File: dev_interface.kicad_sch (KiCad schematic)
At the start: 8 parts, among them U4 ISO164xB, U5 DACx53401, U6 DACx53401, U8 LM2904

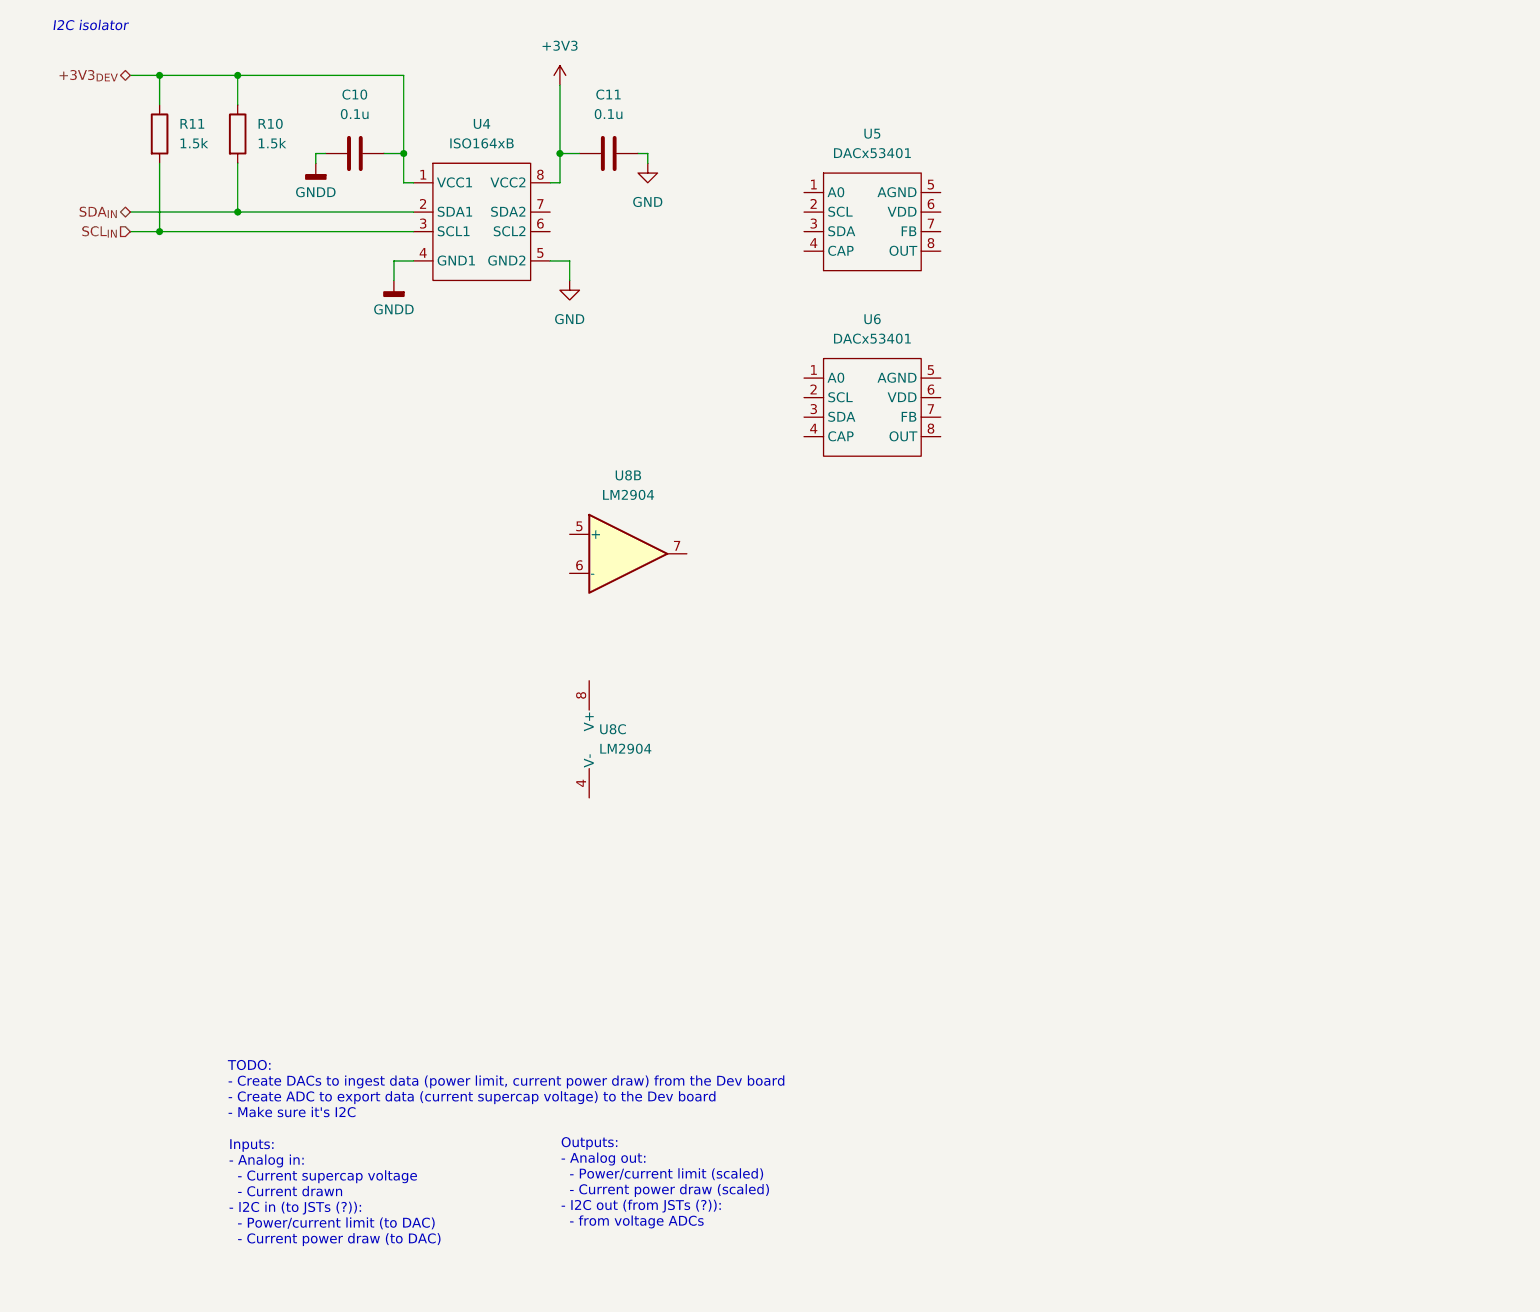
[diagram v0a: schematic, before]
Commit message: Finish Dev board interface
sorry morris
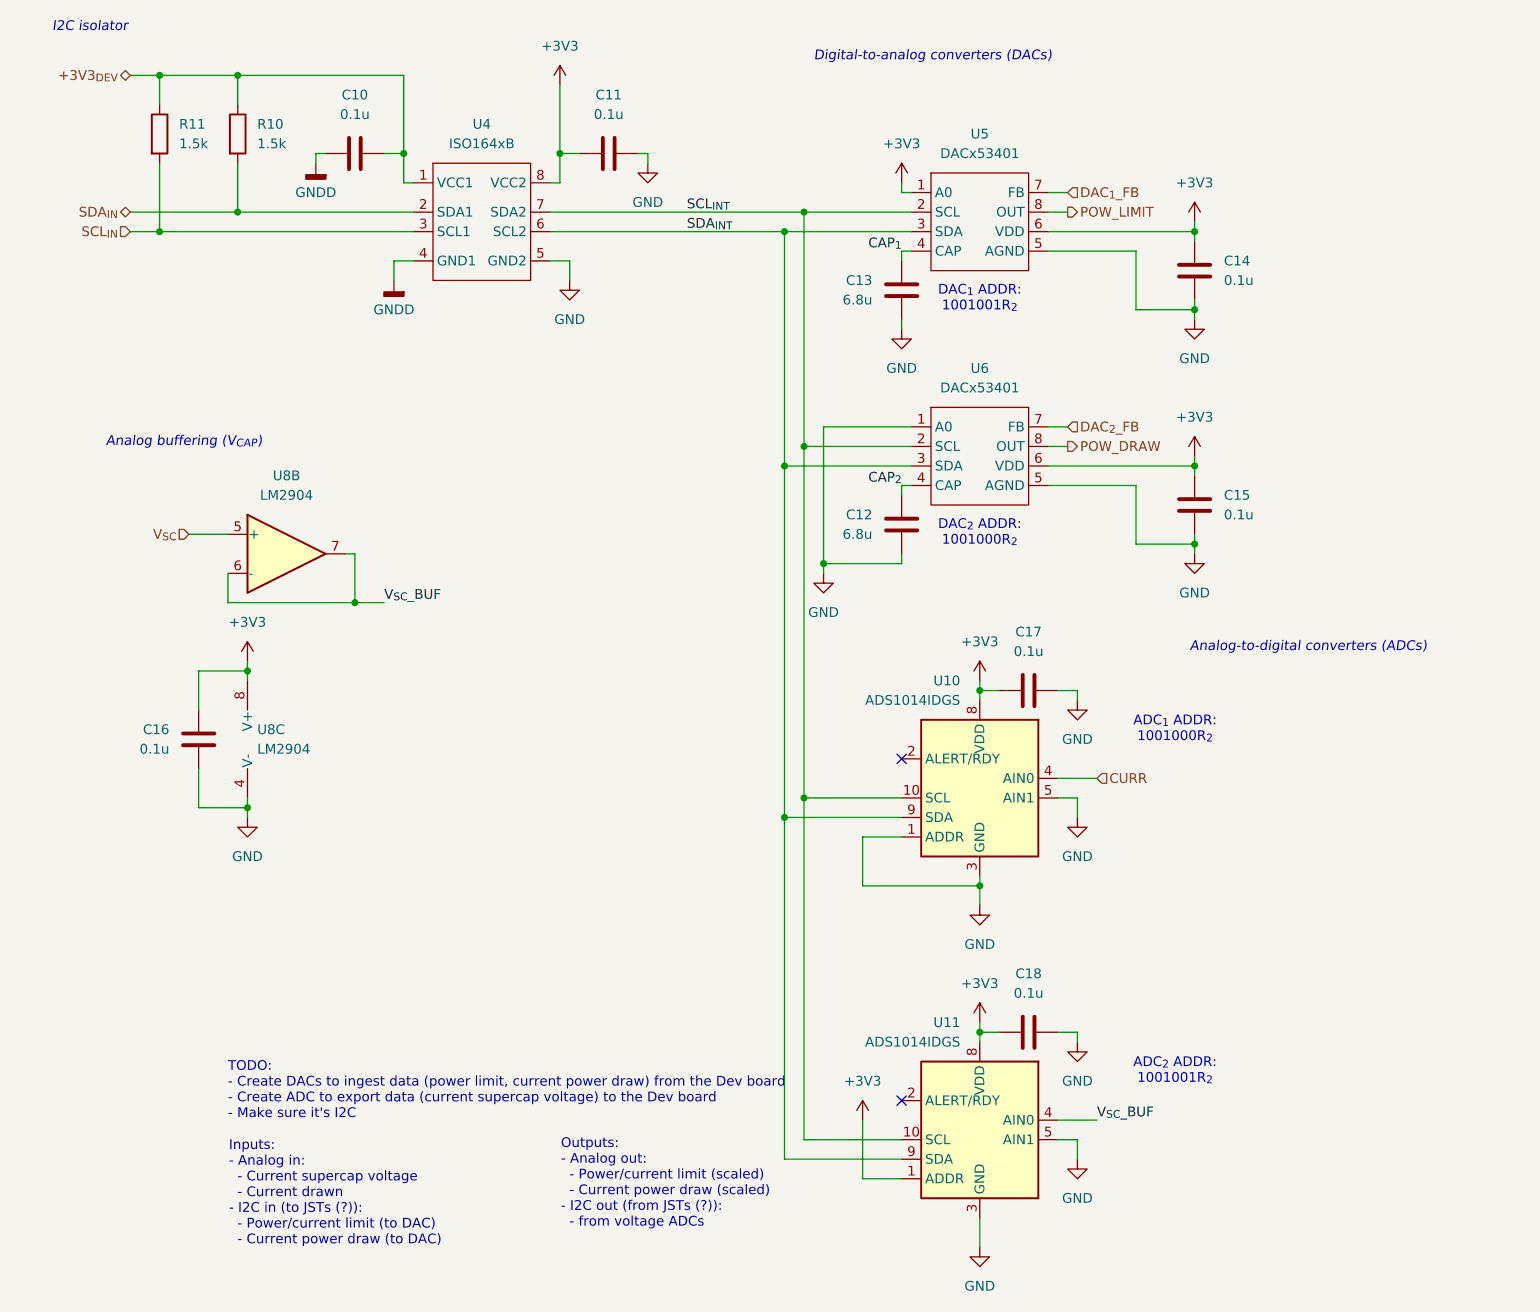
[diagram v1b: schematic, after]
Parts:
- added C12, C13: 6.8u, Capacitor_SMD:C_0603_1608Metric_Pad1.08x0.95mm_HandSolder, symbol Device:C
- added C14, C15, C16, C17, C18: 0.1u, symbol Device:C
- added U10, U11: ADS1014IDGS, Package_SO:TSSOP-10_3x3mm_P0.5mm, symbol Analog_ADC:ADS1014IDGS
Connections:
- net +3V3: now also U5.1 (A0), U5.6 (VDD), U6.6 (VDD), U8.8 (V+), C14.2, C15.2, C16.2, C17.2, C18.2, U10.8 (VDD), U11.1 (ADDR), U11.8 (VDD)
- net GND: now also U5.5 (AGND), U6.1 (A0), U6.5 (AGND), U8.4 (V-), C12.2, C13.2, C14.1, C15.1, C16.1, C17.1, C18.1, U10.1 (ADDR), U10.3 (GND), U10.5 (AIN1), U11.3 (GND), U11.5 (AIN1)
- net SCL_{INT}: now reaches U5.2 (SCL)
- net SCL_{INT}: now also U4.7 (SDA2), U6.2 (SCL), U10.10 (SCL), U11.10 (SCL)
- net SDA_{INT}: now reaches U5.3 (SDA)
- net SDA_{INT}: now also U4.6 (SCL2), U6.3 (SDA), U10.9 (SDA), U11.9 (SDA)
- net CAP_{1}: now reaches U5.4 (CAP)
- net CAP_{1}: now also C13.1
- net DAC_{1}_FB: now reaches U5.7 (FB)
- net POW_LIMIT: now reaches U5.8 (OUT)
- net CAP_{2}: now reaches U6.4 (CAP)
- net CAP_{2}: now also C12.1
- net DAC_{2}_FB: now reaches U6.7 (FB)
- net POW_DRAW: now reaches U6.8 (OUT)
- net V_{SC}: now reaches U8.5 (+)
- net V_{SC}_BUF: now reaches U8.6 (-)
- net V_{SC}_BUF: now also U8.7, U11.4 (AIN0)
- new net CURR: U10.4 (AIN0)
- no-connect marks 0 -> 2
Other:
- note added: "ADC_{1} ADDR: 1001000R_{2}"
- note added: "ADC_{2} ADDR: 1001001R_{2}"
- note added: "Analog buffering (V_{CAP})"
- note added: "Analog-to-digital converters (ADCs)"
- note added: "DAC_{1} ADDR: 1001001R_{2}"
- note added: "DAC_{2} ADDR: 1001000R_{2}"
- note added: "Digital-to-analog converters (DACs)"
- moved on the sheet: U5, U6, U8B, U8C
